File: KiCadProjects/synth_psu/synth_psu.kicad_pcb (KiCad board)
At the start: 2 copper layers, 140.5 x 73 mm, 29 parts, among them J1 Barrel_Jack, J2 Switch Terminals, J3 Output Terminals, J4 Fan 1, J5 Fan 2, U1 LM7815_TO220, U2 LM7915_TO220

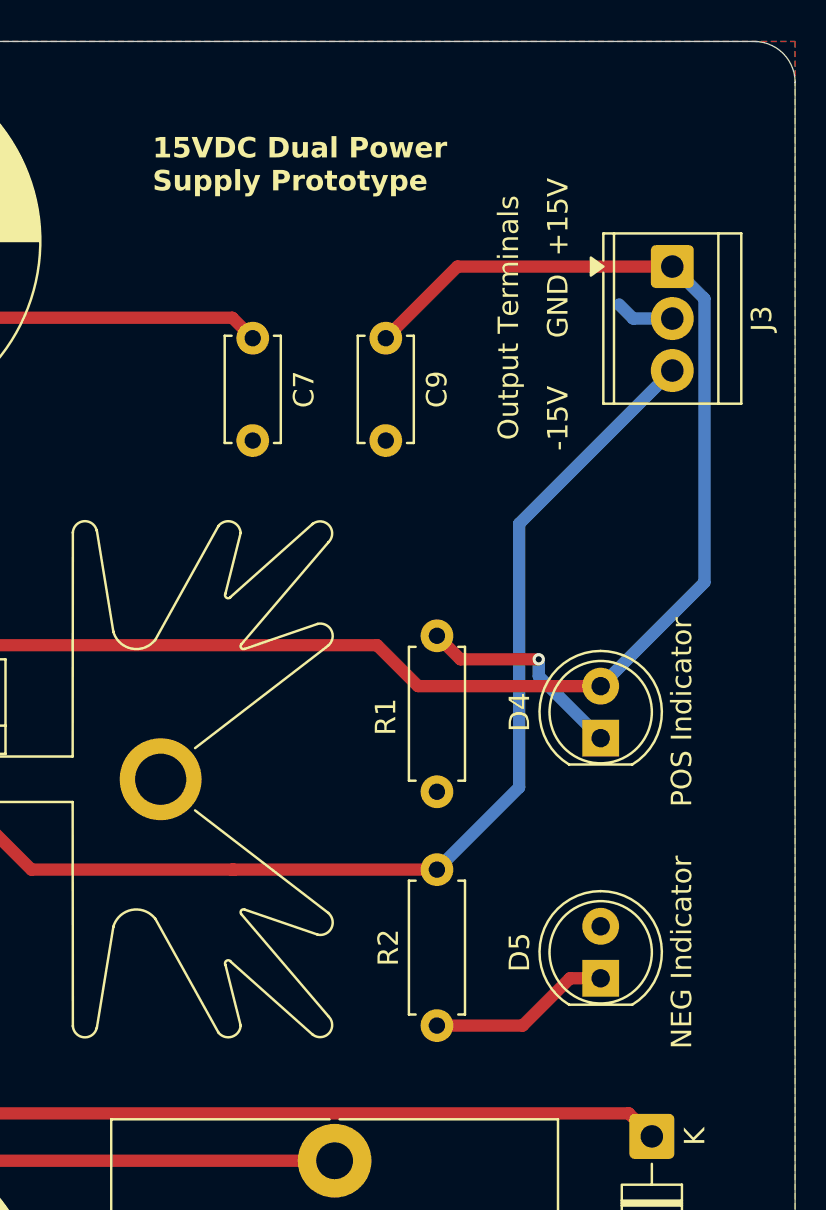
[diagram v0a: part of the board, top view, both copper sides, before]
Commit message: remove old projects
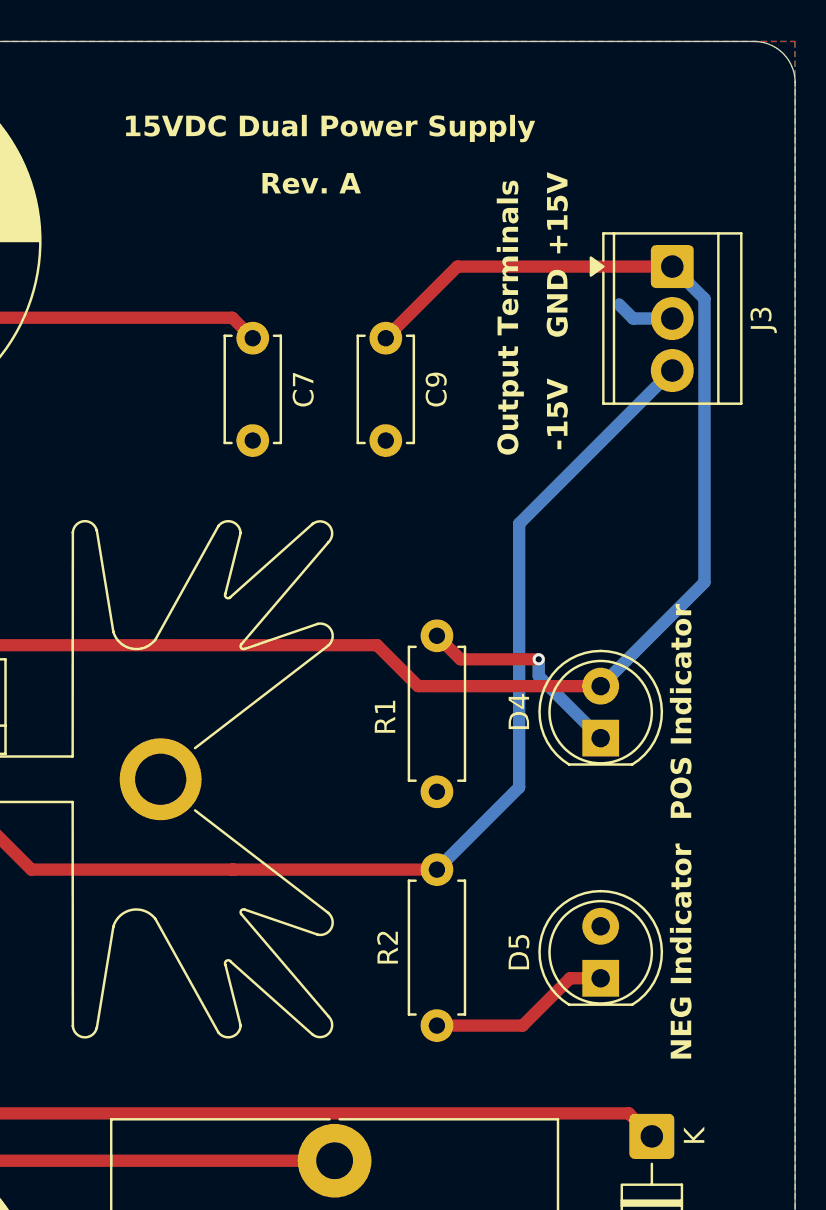
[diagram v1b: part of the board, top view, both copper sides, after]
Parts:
- R1, R2: value 330 -> 1k
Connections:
- J1 pad 3: GND -> (no net)
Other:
- rule pad_to_mask_clearance: 0 -> 0.038
- board text added: "15VDC Dual Power Supply"
- board text added: "Rev. A"
- board text removed: "15VDC Dual Power Supply Prototype"
